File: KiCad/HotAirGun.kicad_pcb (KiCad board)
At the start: 2 copper layers, 49.8 x 17.6 mm, 22 parts, among them J4 Arduino_Nano_Header, Q2 SI2308, SW1 Rotary_Encoder, U1 MAX31855K

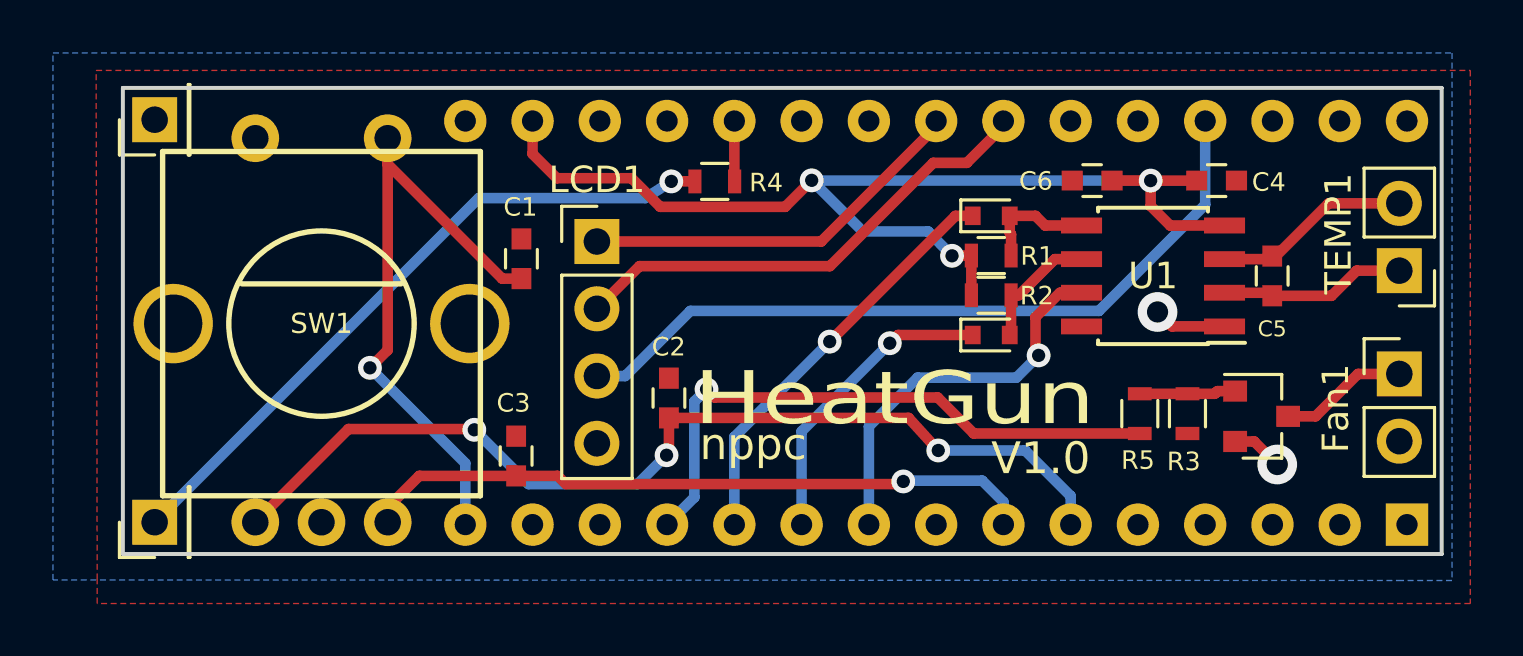
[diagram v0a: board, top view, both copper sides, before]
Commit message: Final adjustments
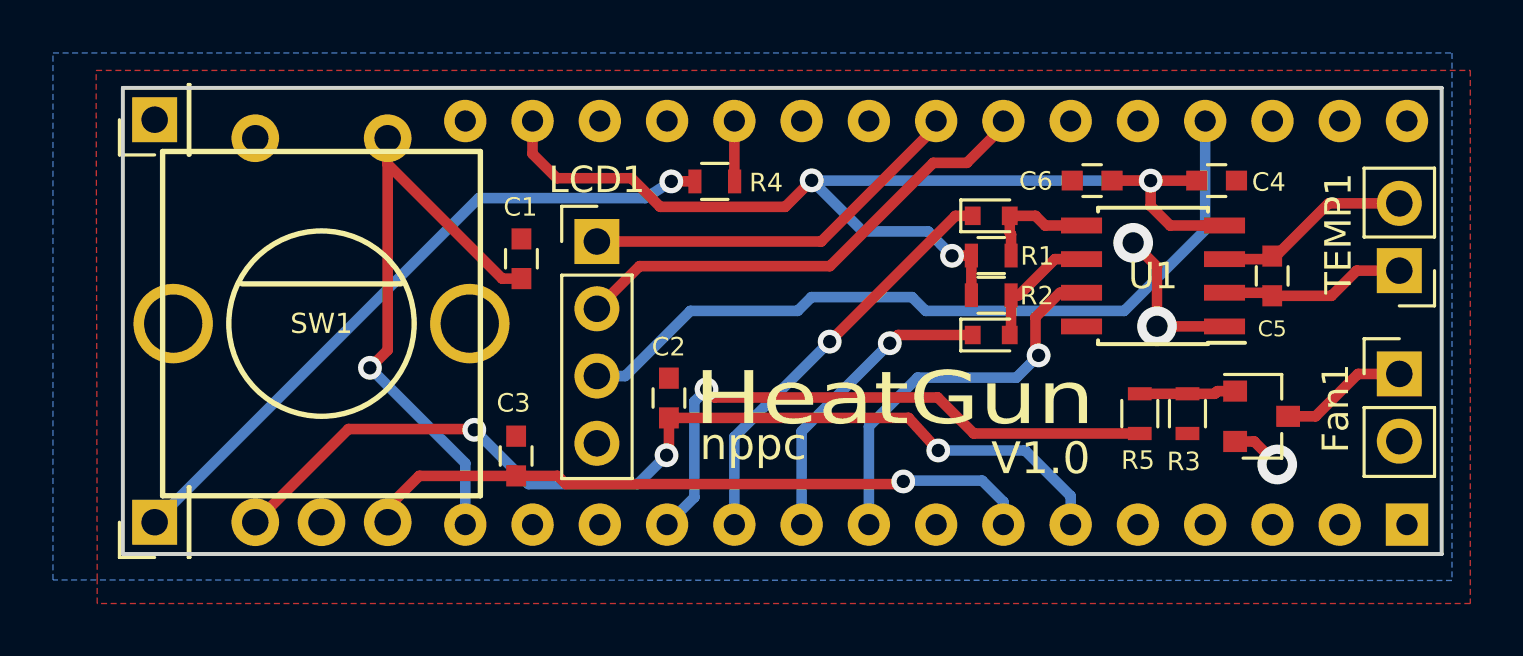
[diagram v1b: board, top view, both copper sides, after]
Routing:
- net GND: track 4.71 -> 8.02 mm, vias 2 -> 3
- net VCC: track 28.8 -> 29.8 mm
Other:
- rule pad_to_mask_clearance: 0.2 -> 0.1
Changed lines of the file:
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@@
     (thickness 1.6)
     (drawings 9)
-    (tracks 148)
+    (tracks 155)
     (zones 0)
     (modules 22)
@@
     (pad_size 1.524 1.524)
     (pad_drill 0.762)
-    (pad_to_mask_clearance 0.2)
+    (pad_to_mask_clearance 0.1)
     (aux_axis_origin 0 0)
     (visible_elements 7FFFFF7F)
@@
   (gr_line (start 173.1 136.1) (end 173.1 118.5) (angle 90) (layer Edge.Cuts) (width 0.15))
   (gr_line (start 123.3 118.5) (end 123.3 136.1) (angle 90) (layer Edge.Cuts) (width 0.15))
+  (segment (start 162.35 127.5) (end 162.35 125.25) (width 0.4) (layer F.Cu) (net 1))
+  (segment (start 162.915 127.505) (end 162.35 127.5) (width 0.4) (layer F.Cu) (net 1))
+  (via (at 162.35 127.5) (size 1.5) (drill 0.8) (layers F.Cu B.Cu) (net 1))
   (segment (start 164.9 127.505) (end 162.915 127.505) (width 0.4) (layer F.Cu) (net 1))
-  (via (at 162.37 126.96) (size 1.5) (drill 0.8) (layers F.Cu B.Cu) (net 1))
-  (segment (start 162.915 127.505) (end 162.37 126.96) (width 0.4) (layer F.Cu) (net 1))
+  (via (at 161.45 124.35) (size 1.5) (drill 0.8) (layers F.Cu B.Cu) (net 1))
+  (segment (start 162.35 125.25) (end 161.45 124.35) (width 0.4) (layer F.Cu) (net 1))
   (segment (start 165.3 131.85) (end 166.02 131.85) (width 0.4) (layer F.Cu) (net 1))
   (via (at 166.89 132.72) (size 1.5) (drill 0.8) (layers F.Cu B.Cu) (net 1))
@@
   (segment (start 155.17 121.33) (end 153.9 121.33) (width 0.4) (layer F.Cu) (net 3))
   (segment (start 156.55 119.4) (end 156.55 119.75) (width 0.4) (layer F.Cu) (net 3))
-  (segment (start 164.17 119.75) (end 164.17 122.91) (width 0.4) (layer B.Cu) (net 4))
-  (segment (start 142.27 129.38) (end 141.2 129.38) (width 0.4) (layer B.Cu) (net 4))
+  (segment (start 144.73 126.92) (end 148.78 126.92) (width 0.4) (layer B.Cu) (net 4))
+  (segment (start 164.17 123.86) (end 161.11 126.92) (width 0.4) (layer B.Cu) (net 4))
   (segment (start 144.73 126.92) (end 142.27 129.38) (width 0.4) (layer B.Cu) (net 4))
-  (segment (start 160.16 126.92) (end 144.73 126.92) (width 0.4) (layer B.Cu) (net 4))
-  (segment (start 164.17 122.91) (end 160.16 126.92) (width 0.4) (layer B.Cu) (net 4))
+  (segment (start 141.2 129.38) (end 142.27 129.38) (width 0.4) (layer B.Cu) (net 4))
+  (segment (start 164.17 123.86) (end 164.17 119.75) (width 0.4) (layer B.Cu) (net 4) (status 800000))
+  (segment (start 153.62 126.92) (end 161.11 126.92) (width 0.4) (layer B.Cu) (net 4))
+  (segment (start 153.1 126.4) (end 153.62 126.92) (width 0.4) (layer B.Cu) (net 4))
+  (segment (start 149.3 126.4) (end 153.1 126.4) (width 0.4) (layer B.Cu) (net 4))
+  (segment (start 148.78 126.92) (end 149.3 126.4) (width 0.4) (layer B.Cu) (net 4))
   (via (at 141.2 129.38) (size 0.9) (drill 0.5) (layers F.Cu B.Cu) (net 4))
   (segment (start 141.2 129.38) (end 141.21 129.39) (width 0.4) (layer B.Cu) (net 4))
